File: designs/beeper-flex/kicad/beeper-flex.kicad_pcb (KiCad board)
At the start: 2 copper layers, 22.2 x 7.9 mm, 7 parts

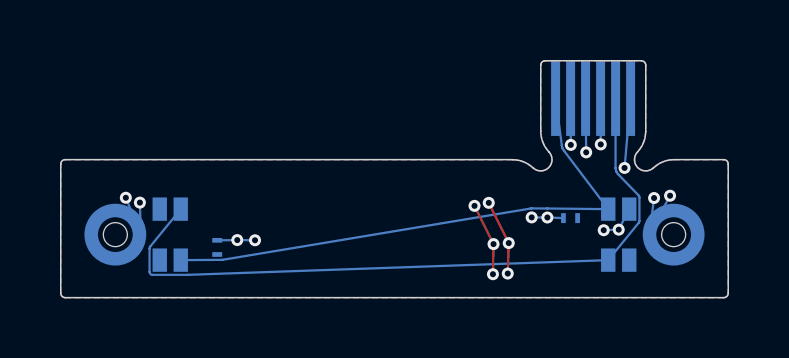
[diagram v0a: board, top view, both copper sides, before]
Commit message: flex to cad with wrong rules
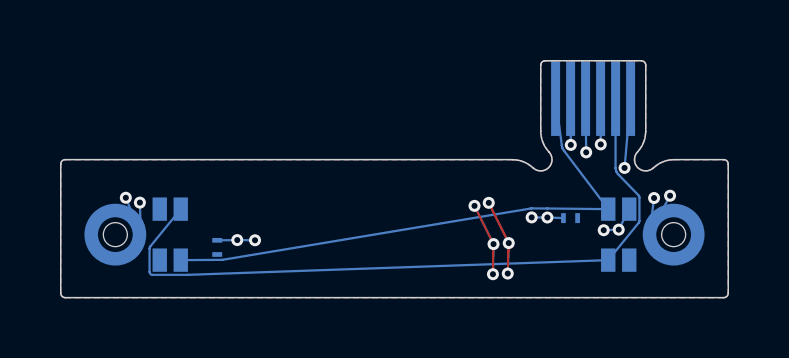
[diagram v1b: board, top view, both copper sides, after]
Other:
- net class Default added: clearance 0.0625, trace_width 0.075, via_dia 0.015, via_drill 0.15
- rule pad_to_mask_clearance: 0 -> 0.051
